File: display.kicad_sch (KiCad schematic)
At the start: 9 parts, among them Q3 BSS138, U8 RS2299XTQC16

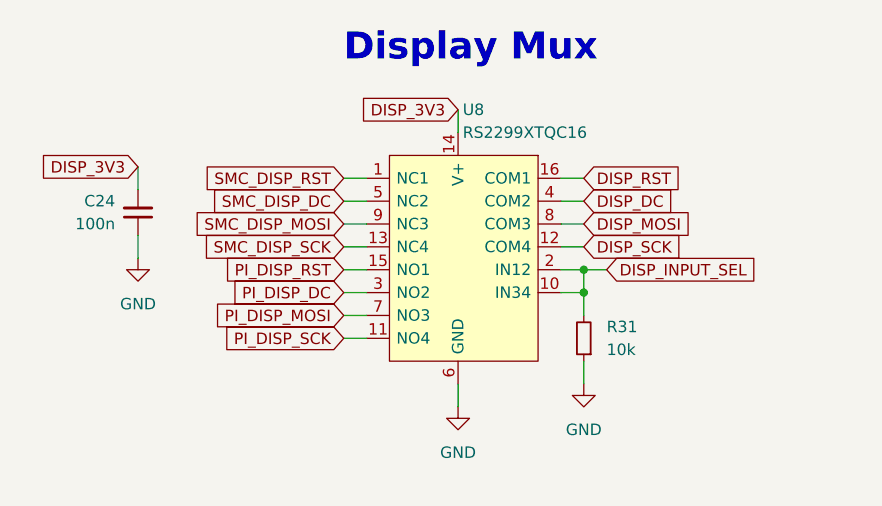
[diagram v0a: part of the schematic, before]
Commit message: routing: begin routing
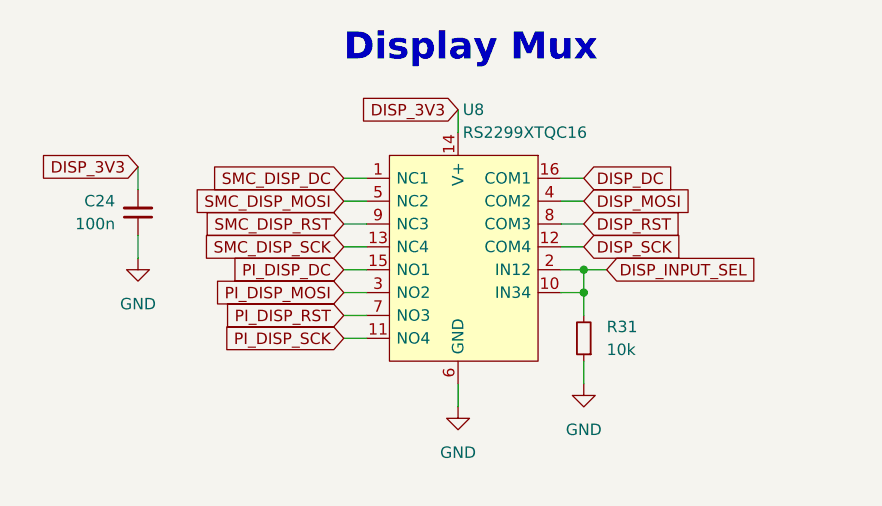
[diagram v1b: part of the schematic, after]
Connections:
- net DISP_DC: now also U8.16 (COM1); no longer U8.4 (COM2)
- net DISP_MOSI: now also U8.4 (COM2); no longer U8.8 (COM3)
- net DISP_RST: now also U8.8 (COM3); no longer U8.16 (COM1)
- net PI_DISP_DC: now also U8.15 (NO1); no longer U8.3 (NO2)
- net PI_DISP_MOSI: now also U8.3 (NO2); no longer U8.7 (NO3)
- net PI_DISP_RST: now also U8.7 (NO3); no longer U8.15 (NO1)
- net SMC_DISP_DC: now also U8.1 (NC1); no longer U8.5 (NC2)
- net SMC_DISP_MOSI: now also U8.5 (NC2); no longer U8.9 (NC3)
- net SMC_DISP_RST: now also U8.9 (NC3); no longer U8.1 (NC1)
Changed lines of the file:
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@@
     )
   )
-  (global_label "SMC_DISP_RST" (shape input) (at 67.31 101.6 180) (fields_autoplaced)
+  (global_label "SMC_DISP_RST" (shape input) (at 67.31 106.68 180) (fields_autoplaced)
     (effects (font (size 1.27 1.27)) (justify right))
-    (property "Intersheet References" "${INTERSHEET_REFS}" (id 0) (at 51.2293 101.5206 0)
+    (property "Intersheet References" "${INTERSHEET_REFS}" (id 0) (at 51.2293 106.6006 0)
       (effects (font (size 1.27 1.27)) (justify right) hide)
     )
@@
     )
   )
-  (global_label "PI_DISP_MOSI" (shape input) (at 67.31 116.84 180) (fields_autoplaced)
+  (global_label "PI_DISP_MOSI" (shape input) (at 67.31 114.3 180) (fields_autoplaced)
     (effects (font (size 1.27 1.27)) (justify right))
-    (property "Intersheet References" "${INTERSHEET_REFS}" (id 0) (at 52.1364 116.7606 0)
+    (property "Intersheet References" "${INTERSHEET_REFS}" (id 0) (at 52.1364 114.2206 0)
       (effects (font (size 1.27 1.27)) (justify right) hide)
     )
   )
-  (global_label "DISP_MOSI" (shape input) (at 93.98 106.68 0) (fields_autoplaced)
+  (global_label "DISP_MOSI" (shape input) (at 93.98 104.14 0) (fields_autoplaced)
     (effects (font (size 1.27 1.27)) (justify left))
-    (property "Intersheet References" "${INTERSHEET_REFS}" (id 0) (at 106.3112 106.6006 0)
+    (property "Intersheet References" "${INTERSHEET_REFS}" (id 0) (at 106.3112 104.0606 0)
       (effects (font (size 1.27 1.27)) (justify left) hide)
     )
   )
-  (global_label "DISP_RST" (shape input) (at 93.98 101.6 0) (fields_autoplaced)
+  (global_label "DISP_RST" (shape input) (at 93.98 106.68 0) (fields_autoplaced)
     (effects (font (size 1.27 1.27)) (justify left))
-    (property "Intersheet References" "${INTERSHEET_REFS}" (id 0) (at 105.1621 101.5206 0)
+    (property "Intersheet References" "${INTERSHEET_REFS}" (id 0) (at 105.1621 106.6006 0)
       (effects (font (size 1.27 1.27)) (justify left) hide)
     )
@@
     )
   )
-  (global_label "SMC_DISP_MOSI" (shape input) (at 67.31 106.68 180) (fields_autoplaced)
+  (global_label "SMC_DISP_MOSI" (shape input) (at 67.31 104.14 180) (fields_autoplaced)
     (effects (font (size 1.27 1.27)) (justify right))
-    (property "Intersheet References" "${INTERSHEET_REFS}" (id 0) (at 50.0802 106.7594 0)
+    (property "Intersheet References" "${INTERSHEET_REFS}" (id 0) (at 50.0802 104.2194 0)
       (effects (font (size 1.27 1.27)) (justify right) hide)
     )
@@
     )
   )
-  (global_label "PI_DISP_RST" (shape input) (at 67.31 111.76 180) (fields_autoplaced)
+  (global_label "PI_DISP_RST" (shape input) (at 67.31 116.84 180) (fields_autoplaced)
     (effects (font (size 1.27 1.27)) (justify right))
-    (property "Intersheet References" "${INTERSHEET_REFS}" (id 0) (at 53.2855 111.6806 0)
+    (property "Intersheet References" "${INTERSHEET_REFS}" (id 0) (at 53.2855 116.7606 0)
       (effects (font (size 1.27 1.27)) (justify right) hide)
     )
@@
     )
   )
-  (global_label "DISP_DC" (shape input) (at 93.98 104.14 0) (fields_autoplaced)
+  (global_label "DISP_DC" (shape input) (at 93.98 101.6 0) (fields_autoplaced)
     (effects (font (size 1.27 1.27)) (justify left))
-    (property "Intersheet References" "${INTERSHEET_REFS}" (id 0) (at 104.255 104.0606 0)
+    (property "Intersheet References" "${INTERSHEET_REFS}" (id 0) (at 104.255 101.5206 0)
       (effects (font (size 1.27 1.27)) (justify left) hide)
     )
   )
-  (global_label "SMC_DISP_DC" (shape input) (at 67.31 104.14 180) (fields_autoplaced)
+  (global_label "SMC_DISP_DC" (shape input) (at 67.31 101.6 180) (fields_autoplaced)
     (effects (font (size 1.27 1.27)) (justify right))
-    (property "Intersheet References" "${INTERSHEET_REFS}" (id 0) (at 52.1364 104.0606 0)
+    (property "Intersheet References" "${INTERSHEET_REFS}" (id 0) (at 52.1364 101.5206 0)
       (effects (font (size 1.27 1.27)) (justify right) hide)
     )
@@
     )
   )
-  (global_label "PI_DISP_DC" (shape input) (at 67.31 114.3 180) (fields_autoplaced)
+  (global_label "PI_DISP_DC" (shape input) (at 67.31 111.76 180) (fields_autoplaced)
     (effects (font (size 1.27 1.27)) (justify right))
-    (property "Intersheet References" "${INTERSHEET_REFS}" (id 0) (at 54.1926 114.2206 0)
+    (property "Intersheet References" "${INTERSHEET_REFS}" (id 0) (at 54.1926 111.6806 0)
       (effects (font (size 1.27 1.27)) (justify right) hide)
     )
